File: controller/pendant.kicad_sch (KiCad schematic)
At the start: 46 parts, among them J1 Conn_01x04_Socket, J2 Conn_01x04_Socket, J3 Conn_01x04_Socket, J4 USB_C_Receptacle_PowerOnly_6P, J5 Conn_01x02_Socket, Q1 BSS138W, Q2 BSS138W, Q3 BSS138W, U1 XC6206P332MR, U2 LIS3DHTR_C15134, U3 STM32C071G8U6, U4 TPS61022, U6 TP4056-42-ESOP8

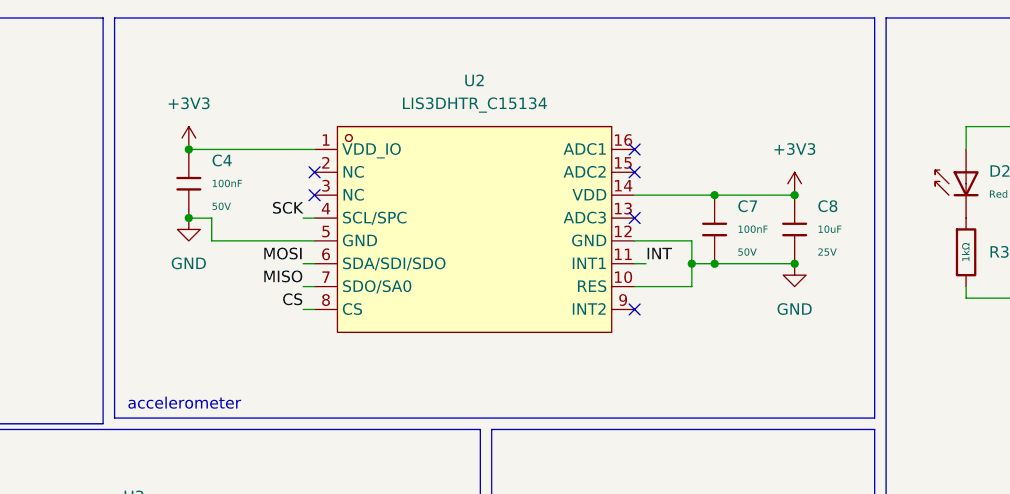
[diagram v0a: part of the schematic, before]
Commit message: feat: other changes
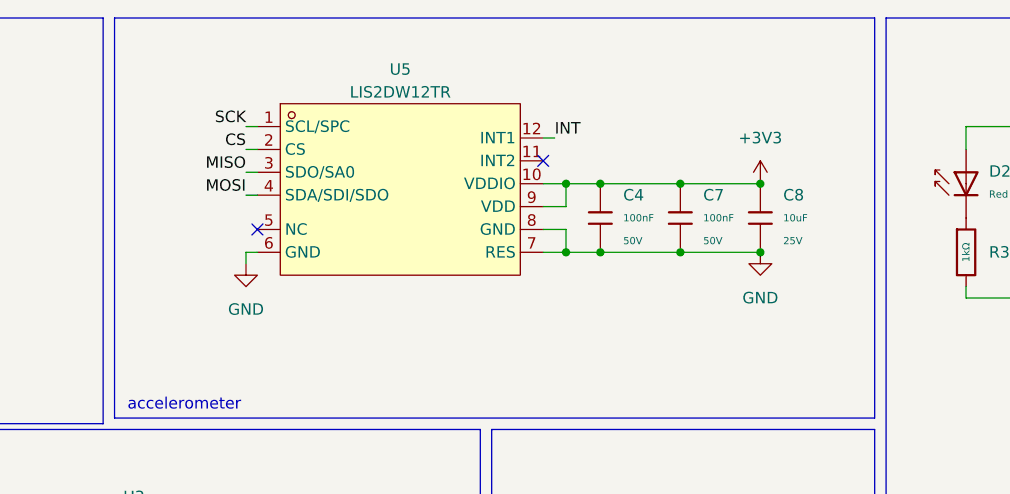
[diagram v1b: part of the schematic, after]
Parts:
- removed U2: LIS3DHTR_C15134, easyeda2kicad:LGA-16_L3.0-W3.0-P0.50-TL, symbol easyeda2kicad:LIS3DHTR_C15134
- added U5: LIS2DW12TR, easyeda2kicad:LGA-12_L2.0-W2.0-P0.50-BL, symbol easyeda2kicad:LIS2DW12TR
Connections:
- net +3V3: now also C4.2, U5.10 (VDDIO), U5.9 (VDD); no longer C4.1
- net CS: now also U5.2 (CS)
- net GND: now also C4.1, U5.6 (GND), U5.7 (RES), U5.8 (GND); no longer C4.2
- net INT: now also U5.12 (INT1)
- net MISO: now also U5.3 (SDO/SA0)
- net MOSI: now also U5.4 (SDA/SDI/SDO)
- net SCK: now also U5.1 (SCL/SPC)
- no-connect marks 9 -> 5
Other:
- moved on the sheet: C4, C7, C8
